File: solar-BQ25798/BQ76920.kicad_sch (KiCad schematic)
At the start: 33 parts, among them Q1801 CSD17578Q3A, Q1802 Q_PMOS_GSD, Q1803 CSD17578Q3A, U1801 BQ76920PW

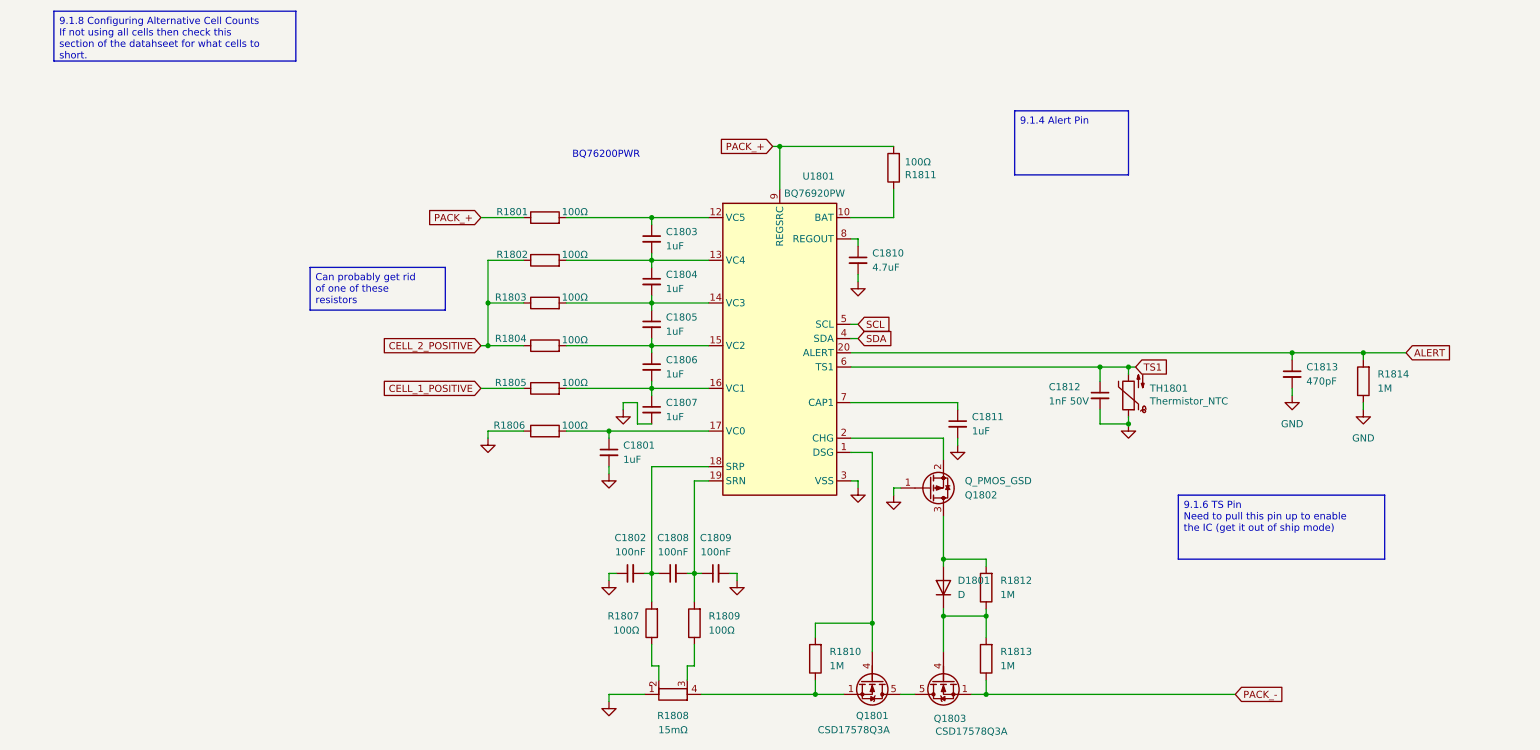
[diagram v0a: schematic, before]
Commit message: Tidy up
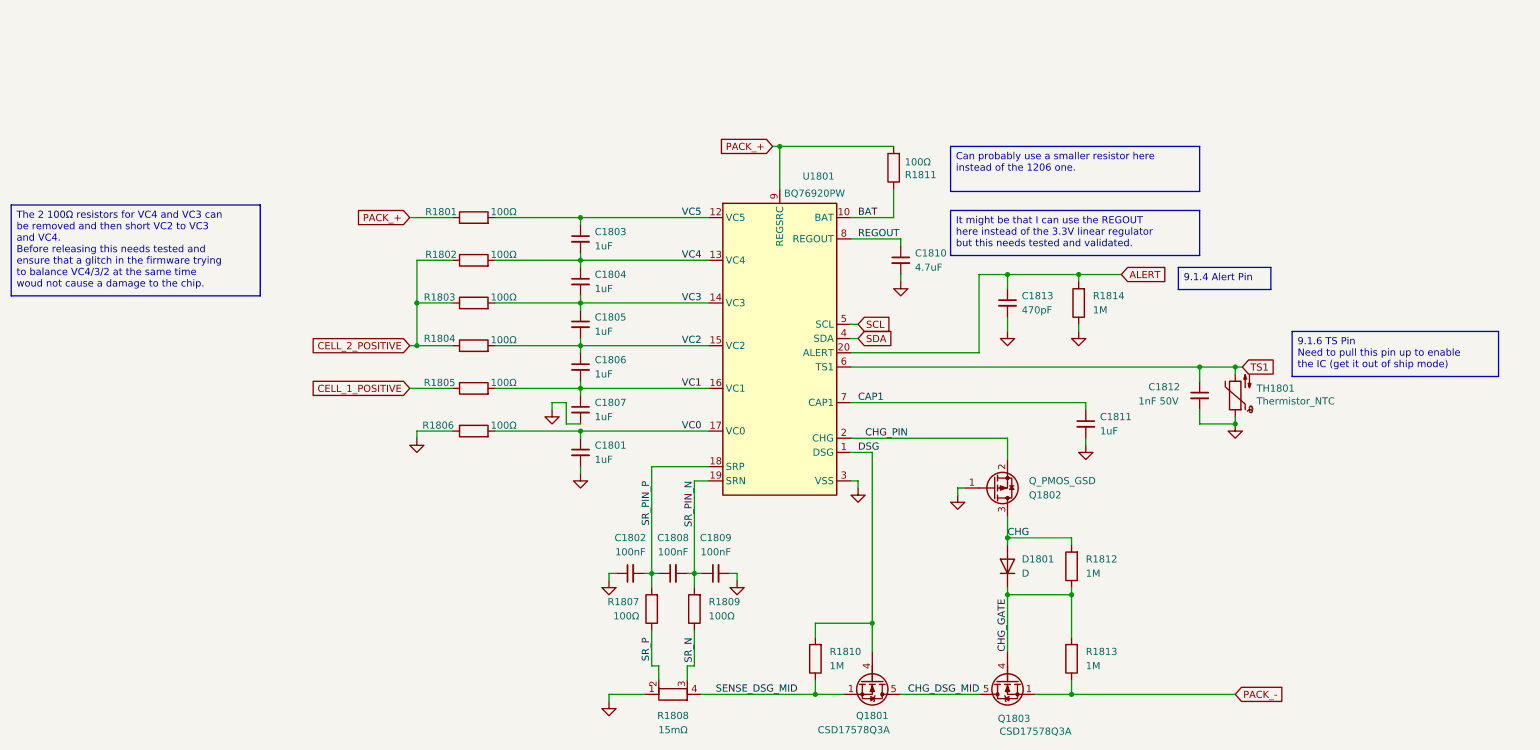
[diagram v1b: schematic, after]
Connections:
- net SR_PIN_N: now reaches C1808.2, C1809.1, R1809.2, U1801.19 (SRN)
- net VC2: now reaches C1805.2, C1806.1, R1804.2, U1801.15 (VC2)
- net SR_N: now reaches R1808.3, R1809.1
- net SR_PIN_P: now reaches C1802.2, C1808.1, R1807.2, U1801.18 (SRP)
- net VC0: now reaches C1801.1, R1806.2, U1801.17 (VC0)
- net VC1: now reaches C1806.2, C1807.1, R1805.2, U1801.16 (VC1)
- net CHG_GATE: now reaches D1801.1 (K), Q1803.4 (G), R1812.1, R1813.2
- net CHG: now reaches D1801.2 (A), Q1802.3 (D), R1812.2
- net BAT: now reaches R1811.1, U1801.10 (BAT)
- net VC4: now reaches C1803.2, C1804.1, R1802.2, U1801.13 (VC4)
- net VC3: now reaches C1804.2, C1805.1, R1803.2, U1801.14 (VC3)
- net CHG_PIN: now reaches Q1802.2 (S), U1801.2 (CHG)
- net SENSE_DSG_MID: now reaches Q1801.1 (S), Q1801.2 (S), Q1801.3 (S), R1808.4, R1810.1
- net DSG: now reaches Q1801.4 (G), R1810.2, U1801.1 (DSG)
- net CHG_DSG_MID: now reaches Q1801.5 (D), Q1803.5 (D)
- net VC5: now reaches C1803.1, R1801.2, U1801.12 (VC5)
- net SR_P: now reaches R1807.1, R1808.2
- net REGOUT: now reaches C1810.1, U1801.8 (REGOUT)
- net CAP1: now reaches C1811.1, U1801.7 (CAP1)
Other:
- note removed: "BQ76200PWR"
- moved on the sheet: C1801, C1803, C1804, C1805, C1806, C1807, C1810, C1811, C1812, C1813, D1801, Q1802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
